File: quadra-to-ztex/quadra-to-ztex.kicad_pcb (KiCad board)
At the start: 4 copper layers, 100 x 100 mm, 33 parts, among them IC1 74CB3T16211DGGR, IC2 74CB3T16211DGGR, IC3 74CB3T16211DGGR, IC4 74CB3T16211DGGR, J1 Conn_02x07_Odd_Even, J2 10029449-111RLF (HDMI A), J3 A2541HWR-2x6P (Pmod 2x6 F R), U1 TPD12S016PWR, U14 8807-140-170LH

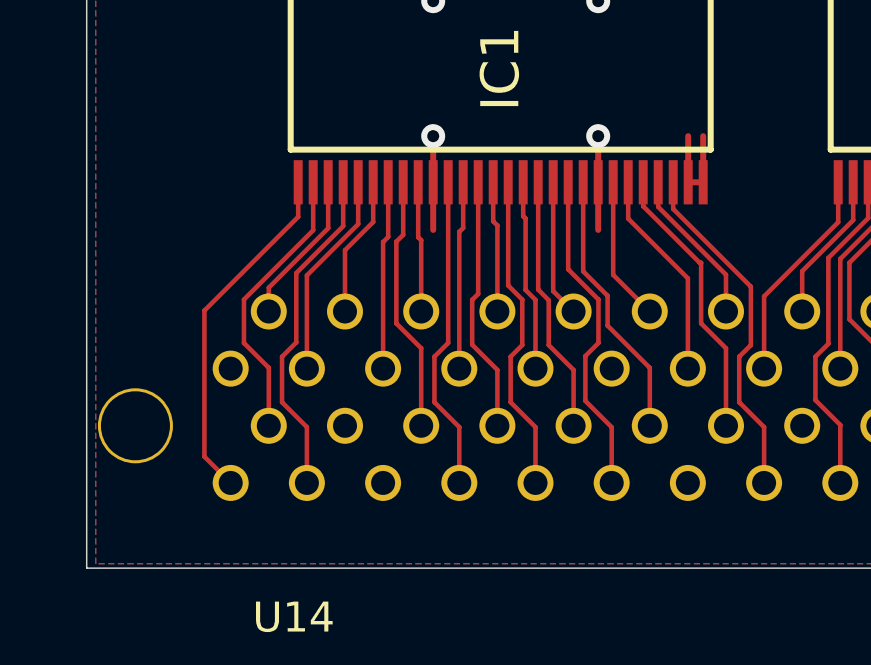
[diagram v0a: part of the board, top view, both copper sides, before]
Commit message: oups A5
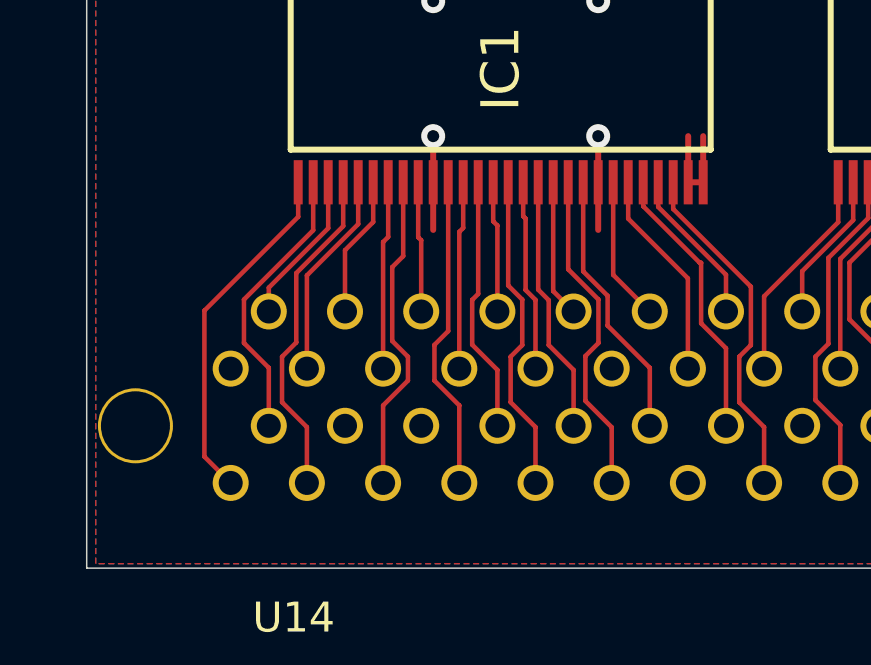
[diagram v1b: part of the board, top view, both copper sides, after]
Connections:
- U14 pad 75: GND -> A5
- U14 pad 76: A5 -> GND
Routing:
- net A5: track 8.55 -> 10.7 mm

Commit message: regen
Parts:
- IC1, IC2, IC3, IC4: footprint For_SeeedStudio:SOP50P810X120-56N -> SOP50P810X120-56N
